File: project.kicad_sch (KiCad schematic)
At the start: 3 parts, among them U1 WLC1115-68LQXQ

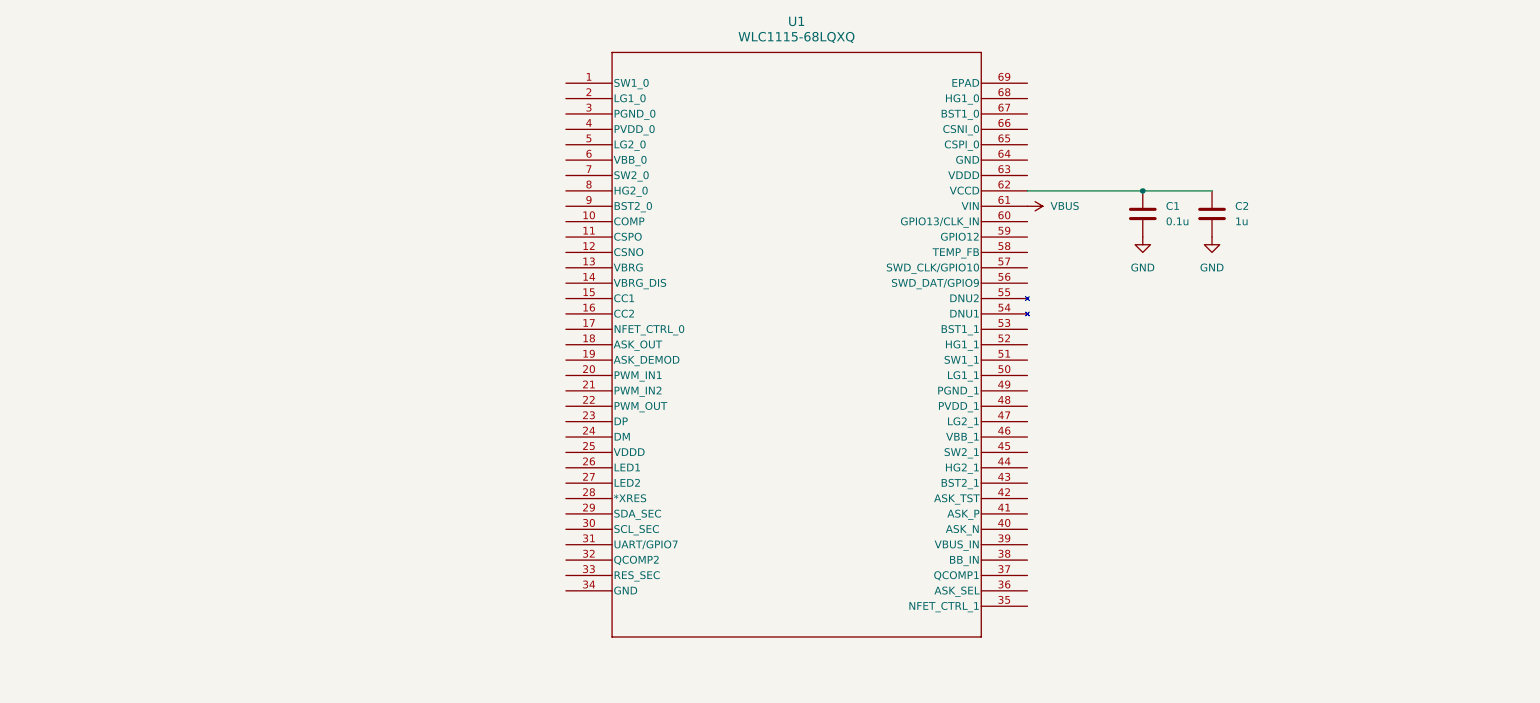
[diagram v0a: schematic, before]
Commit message: started schem
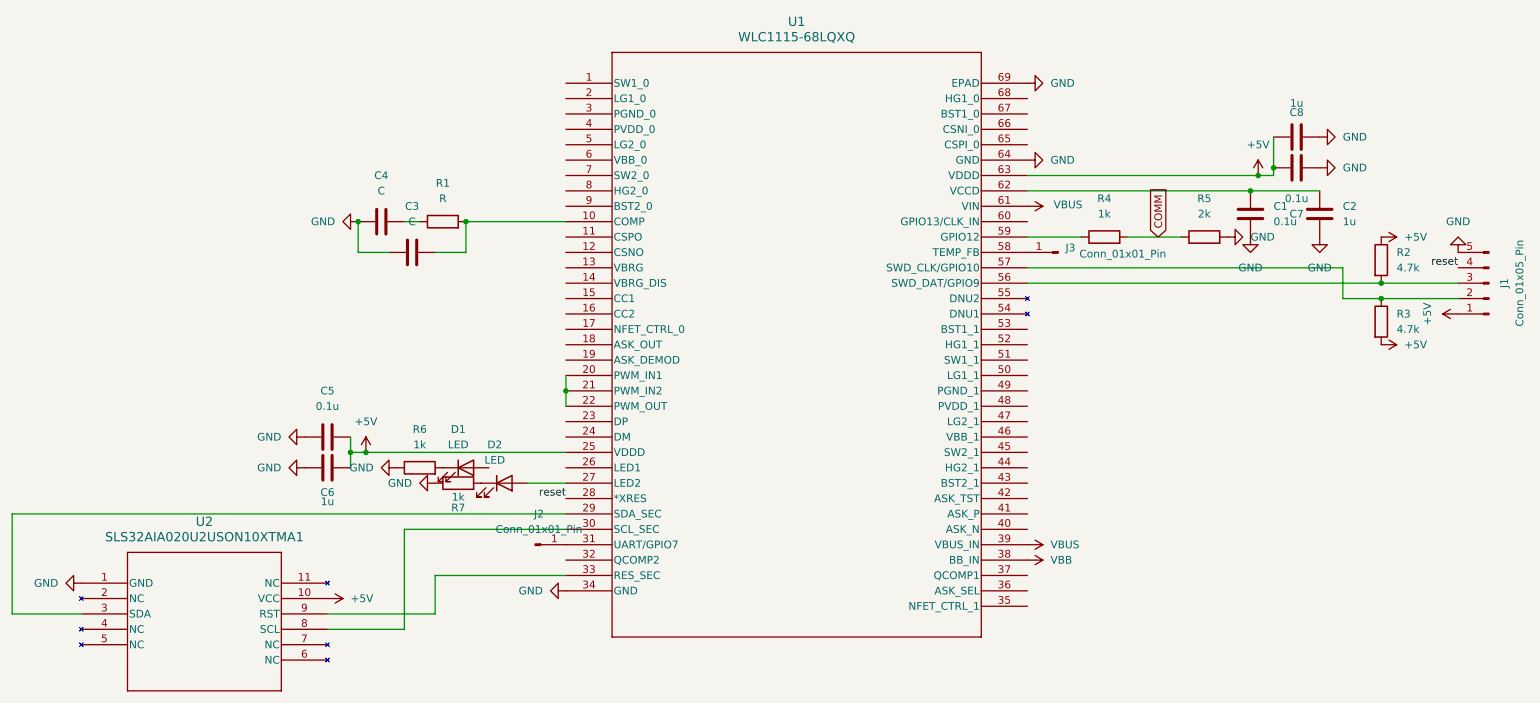
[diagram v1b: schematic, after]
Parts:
- added C3, C4: C, symbol Device:C
- added C5, C7: 0.1u, symbol Device:C
- added C6, C8: 1u, symbol Device:C
- added D1, D2: LED, symbol Device:LED
- added J1: Conn_01x05_Pin, symbol Connector:Conn_01x05_Pin
- added J2, J3: Conn_01x01_Pin, symbol Connector:Conn_01x01_Pin
- added R1: R, symbol Device:R
- added R2, R3: 4.7k, symbol Device:R
- added R4, R6, R7: 1k, symbol Device:R
- added R5: 2k, symbol Device:R
- added U2: SLS32AIA020U2USON10XTMA1, PG-USON-10-2, symbol Optiga Trust:SLS32AIA020U2USON10XTMA1
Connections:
- net GND: now also U1.34 (GND), U1.64 (GND), U1.69 (EPAD), C3.1, C4.1, C5.1, C6.1, C7.1, C8.1, J1.5 (Pin_5), R5.2, R6.1, R7.1, U2.1 (GND)
- net VBUS: now also U1.39 (VBUS_IN)
- net at U1.10 (COMP): now also C3.2, R1.2
- net at U1.20 (PWM_IN1): now also U1.21 (PWM_IN2), U1.22 (PWM_OUT)
- net +5V: now reaches U1.25 (VDDD)
- net +5V: now also U1.63 (VDDD), C5.2, C6.2, C7.2, C8.2, J1.1 (Pin_1), R2.1, R3.2, U2.10 (VCC)
- net at U1.27 (LED2): now also D2.2 (A)
- net reset: now reaches U1.28 (*XRES)
- net reset: now also J1.4 (Pin_4)
- net at U1.29 (SDA_SEC): now also U2.3 (SDA)
- net at U1.30 (SCL_SEC): now also U2.8 (SCL)
- net at U1.31 (UART/GPIO7): now also J2.1 (Pin_1)
- net at U1.33 (RES_SEC): now also U2.9 (RST)
- net VBB: now reaches U1.38 (BB_IN)
- net at U1.56 (SWD_DAT/GPIO9): now also J1.3 (Pin_3), R2.2
- net at U1.57 (SWD_CLK/GPIO10): now also J1.2 (Pin_2), R3.1
- net at U1.58 (TEMP_FB): now also J3.1 (Pin_1)
- net at U1.59 (GPIO12): now also R4.1
- new net: D2.1 (K), R7.2
- new net: C4.2, R1.1
- new net: D1.1 (K), R6.2
- new net COMM: R4.2, R5.1
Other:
- moved on the sheet: C1, C2
